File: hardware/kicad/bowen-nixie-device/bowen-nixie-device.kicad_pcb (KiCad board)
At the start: 2 copper layers, 29.2 x 29.2 mm, 119 parts, among them J1 Conn_01x02_Pin, J2 Conn_01x02_Pin, J3 Conn_01x04_Pin, Q1 SS8050, Q10 MMBTA42, Q11 MMBTA42, Q12 MMBTA42, Q13 MMBTA42, Q14 MMBTA42, Q15 MMBTA42, Q16 MMBTA42, Q17 MMBTA42, Q18 MMBTA42, Q19 MMBTA42, Q2 MPSA92, Q20 MMBTA42, Q21 MMBTA42, Q22 MMBTA42, Q23 MMBTA42, Q24 MMBTA42, Q25 MMBTA42, Q26 MMBTA42, Q27 MMBTA42, Q28 MMBTA42, Q29 MMBTA42, Q3 SS8050, Q30 MMBTA42, Q31 MMBTA42, Q32 MMBTA42, Q33 MMBTA42, Q34 MMBTA42, Q35 MMBTA42, Q36 MMBTA42, Q37 MMBTA42, Q38 MMBTA42, Q39 MMBTA42, Q4 MPSA92, Q40 MMBTA42, Q41 MMBTA42, Q42 MMBTA42, Q43 MMBTA42, Q44 MMBTA42, Q45 MMBTA42, Q46 MMBTA42, Q47 MMBTA42, Q48 MMBTA42, Q5 SS8050, Q6 MPSA92, Q7 SS8050, Q8 MPSA92, Q9 MMBTA42, U1 MOUDLE-SEEEDUINO-XIAO-ESP32C3, U11 NCH8200HV, U2 74HC595, U3 74HC595, U4 74HC595, U5 74HC595, U6 74HC595

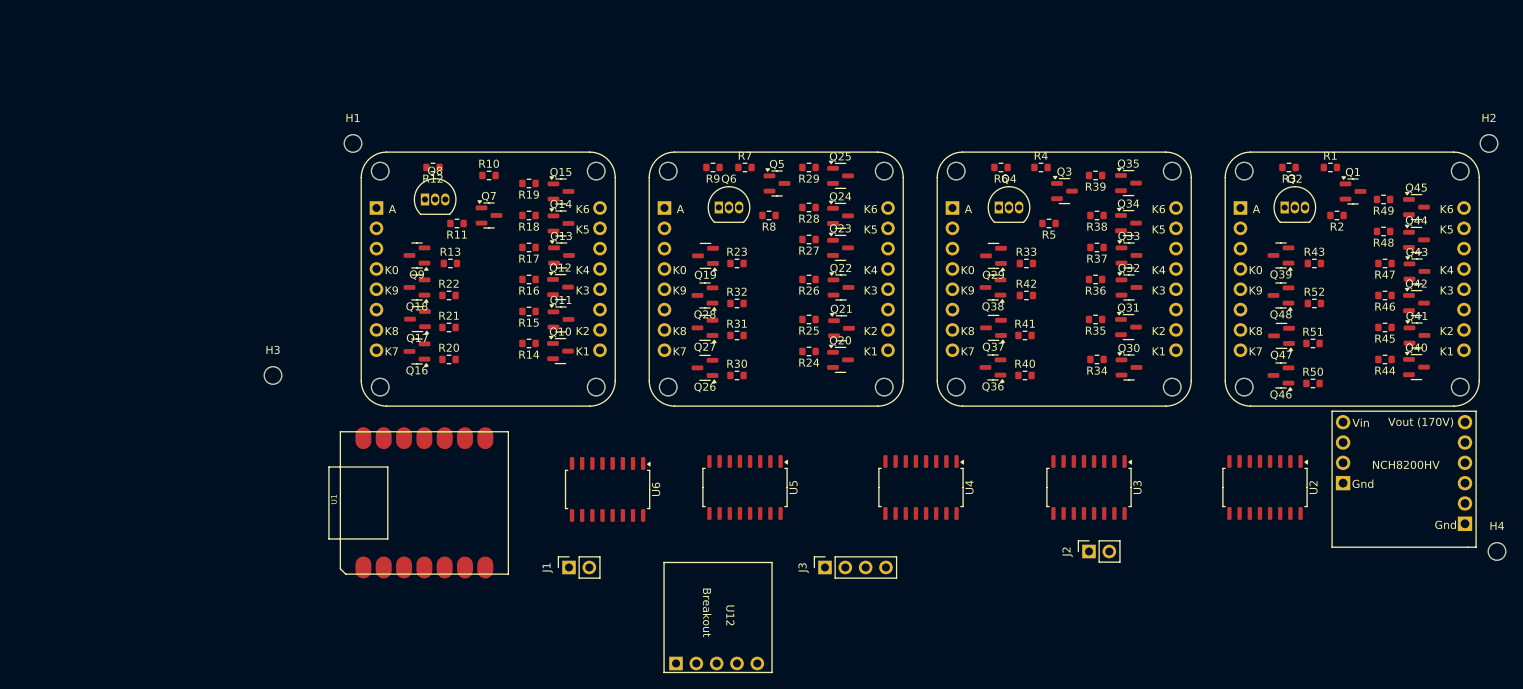
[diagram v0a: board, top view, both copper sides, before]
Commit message: bowen progress
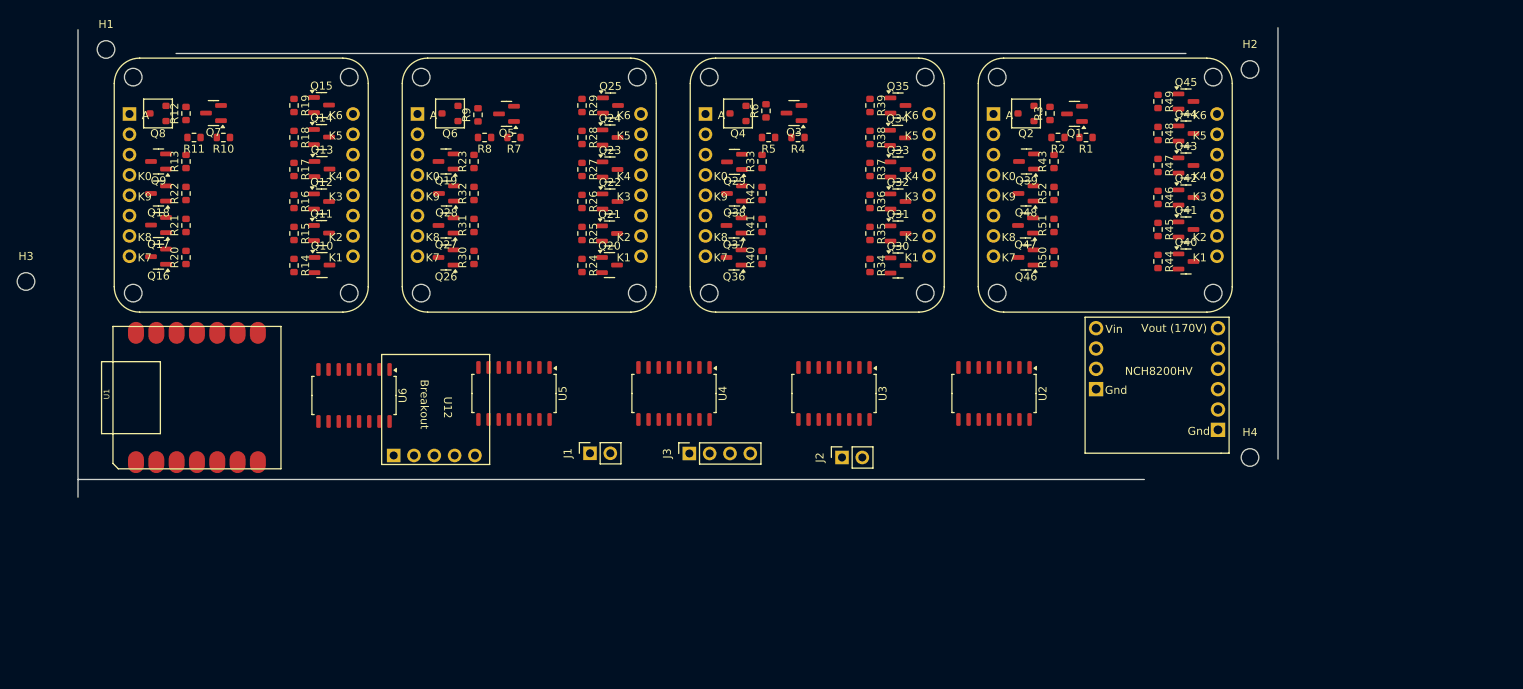
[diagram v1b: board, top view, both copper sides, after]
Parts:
- Q1, Q3, Q5, Q7: value SS8050 -> MMBTA42
- Q2, Q4, Q6, Q8: value MPSA92 -> MMBTA92; footprint Package_TO_SOT_THT:TO-92_Inline -> PCM_Package_TO_SOT_SMD_AKL:SOT-23
- moved U12 43.8 mm to (95.3, 94.2)
- moved R8 36.9 mm to (101.5, 60.2)
- moved Q7 36.7 mm to (67.6, 57.2), turned to 180 degrees
- moved R5 36.7 mm to (136.9, 60.2)
- moved R2 36.2 mm to (173.1, 60.2)
- moved Q1 36.1 mm to (175.2, 57.3), turned to 180 degrees
- moved R30 36.0 mm to (100.1, 75.2), turned to 90 degrees
- moved R40 36.0 mm to (136.1, 75.2), turned to 90 degrees
- moved R50 36.0 mm to (172.6, 75.2), turned to 90 degrees
- moved U2 35.9 mm to (165.1, 92.2)
- moved R31 35.6 mm to (100.1, 71.2), turned to 90 degrees
- moved R32 35.6 mm to (100.1, 67.2), turned to 90 degrees
- moved R41 35.6 mm to (136.1, 71.2), turned to 90 degrees
- moved Q6 35.6 mm to (97.1, 57.2), turned to 180 degrees
- moved R51 35.6 mm to (172.6, 71.2), turned to 90 degrees
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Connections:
- Q2 pad 1: 170V -> Net-(Q2-E)
- Q2 pad 2: Net-(Q2-B) -> 170V
- Q4 pad 1: 170V -> Net-(Q4-E)
- Q4 pad 2: Net-(Q4-B) -> 170V
- Q6 pad 1: 170V -> Net-(Q6-E)
- Q6 pad 2: Net-(Q6-B) -> 170V
- Q8 pad 1: 170V -> Net-(Q8-B)
- Q8 pad 2: Net-(Q8-B) -> 170V
- R2 pad 2: Net-(Q2-B) -> Net-(Q2-E)
- R3 pad 1: Net-(Q2-B) -> Net-(Q2-E)
- R5 pad 2: Net-(Q4-B) -> Net-(Q4-E)
- R6 pad 1: Net-(Q4-B) -> Net-(Q4-E)
- R8 pad 2: Net-(Q6-B) -> Net-(Q6-E)
- R9 pad 1: Net-(Q6-B) -> Net-(Q6-E)
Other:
- board size 29.2 x 29.2 mm -> 150 x 58.7 mm

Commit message: bowen layout progress
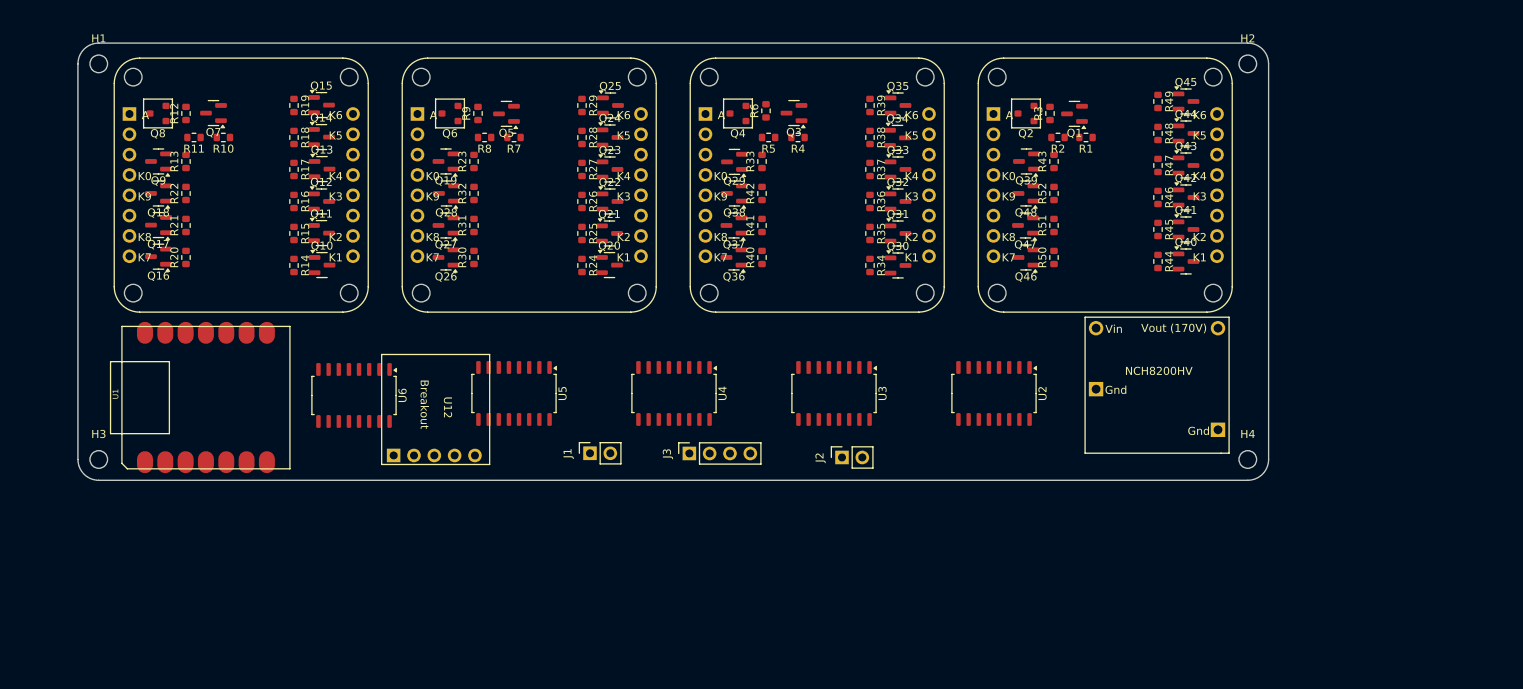
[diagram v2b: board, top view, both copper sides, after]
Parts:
- moved H3 24.0 mm to (53.2, 100.5)
- moved H1 2.01 mm to (53.2, 51.0)
- moved U1 1.12 mm to (77.1, 101.7)
- moved H2 0.75 mm to (196.8, 51.0)
- moved H4 0.37 mm to (196.8, 100.5)
- moved R9 0.17 mm to (100.6, 57.2)
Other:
- board size 150 x 58.7 mm -> 148.8 x 54.6 mm
